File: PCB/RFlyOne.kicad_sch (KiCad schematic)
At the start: 21 parts, among them J1 UFL, Q1 AO3401A, U1 TQP3M9036, U2 TLV3201AIDBVR, U3 TA0970A, U4 TQP3M9036, U5 TA0970A

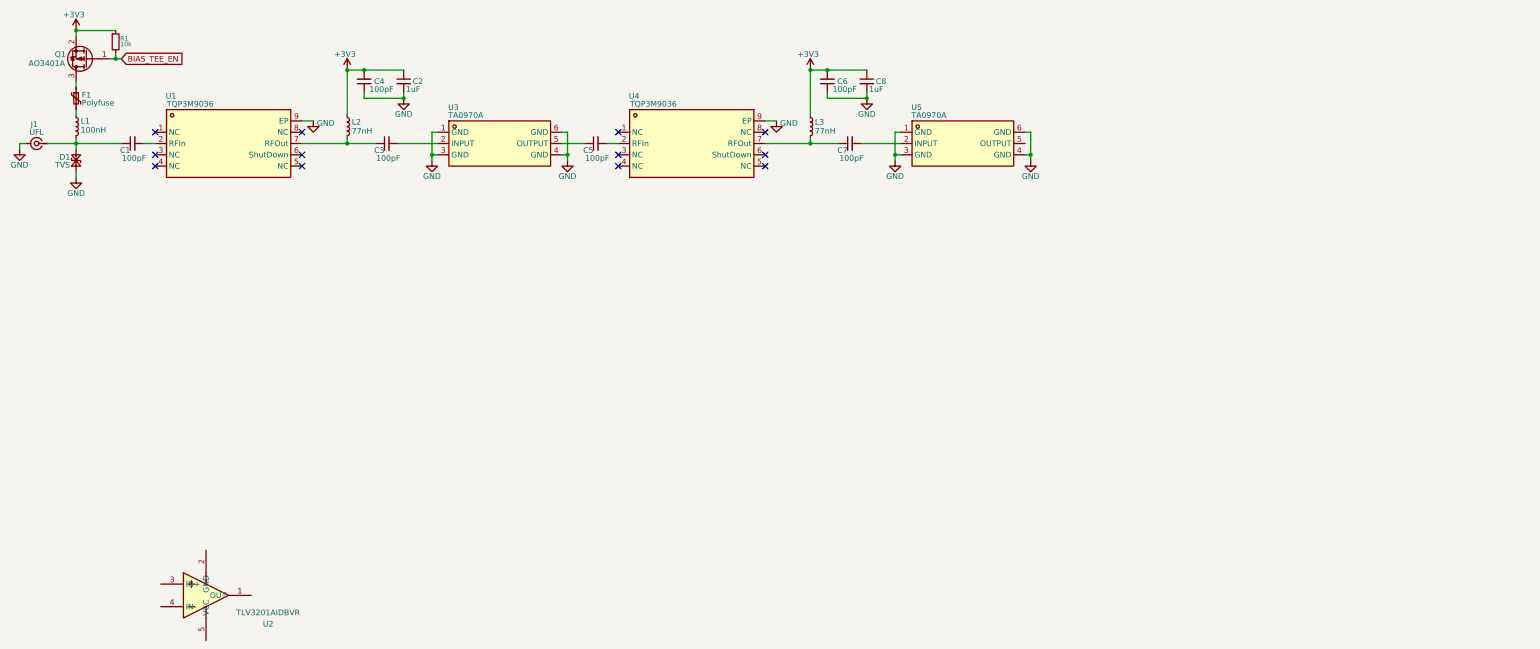
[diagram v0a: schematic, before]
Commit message: checkpoint
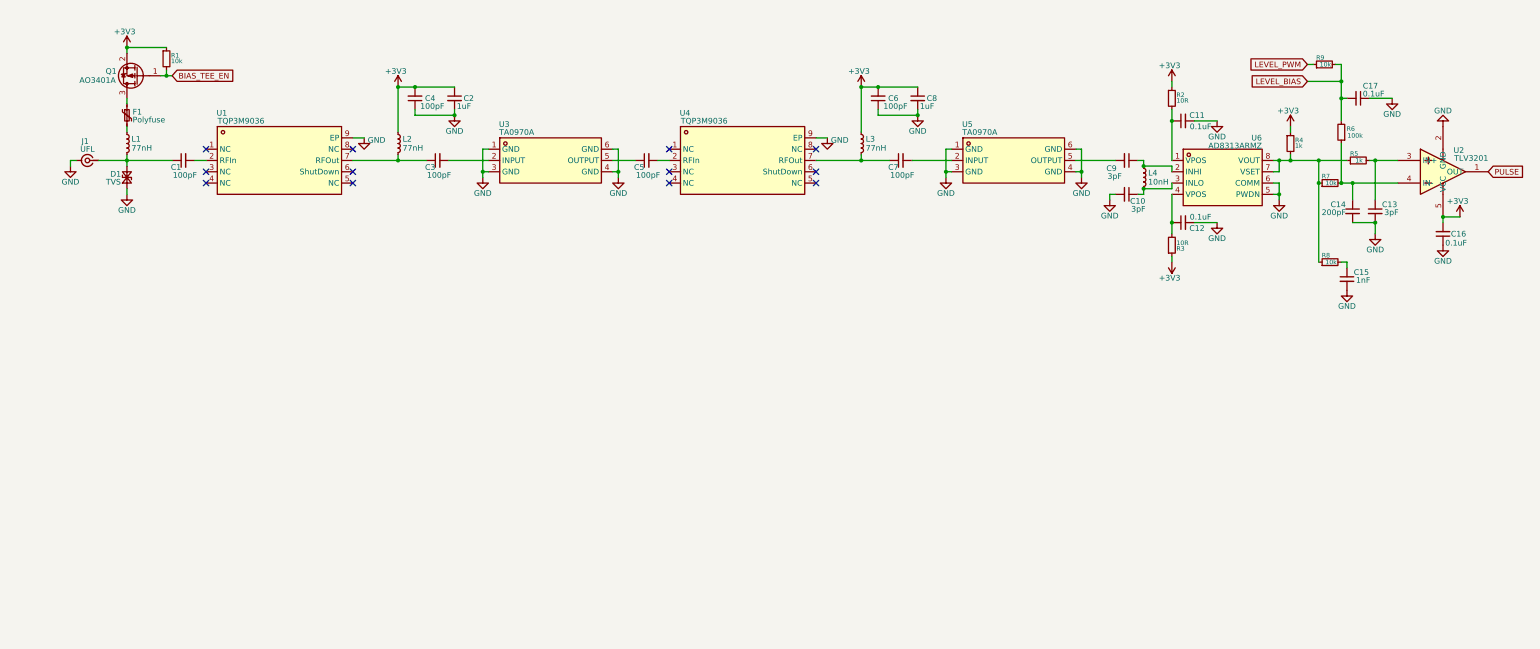
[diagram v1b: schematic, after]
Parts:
- added C10, C13, C9: 3pF, Capacitor_SMD:C_0402_1005Metric, symbol Device:C_Small
- added C11, C12, C16, C17: 0.1uF, Capacitor_SMD:C_0402_1005Metric, symbol Device:C_Small
- added C14: 200pF, Capacitor_SMD:C_0402_1005Metric, symbol Device:C_Small
- added C15: 1nF, Capacitor_SMD:C_0402_1005Metric, symbol Device:C_Small
- added L4: 10nH, Inductor_SMD:L_0402_1005Metric, symbol Device:L_Small
- added R2, R3: 10R, Resistor_SMD:R_0402_1005Metric, symbol Device:R_Small
- added R4, R5: 1k, Resistor_SMD:R_0402_1005Metric, symbol Device:R_Small
- added R6: 100k, Resistor_SMD:R_0402_1005Metric, symbol Device:R_Small
- added R7, R8, R9: 10k, Resistor_SMD:R_0402_1005Metric, symbol Device:R_Small
- added U6: AD8313ARMZ, easyeda2kicad:MSOP-8_L3.0-W3.0-P0.65-LS4.9-BL, symbol RFlyOne:AD8313ARMZ
- C1, C3, C4, C5, C6, C7: LCSC Part C1546 -> C77177
- L1: value 100nH -> 77nH; footprint easyeda2kicad:IND-SMD_L1.8-W1.2_LCF0603-150J-T -> Inductor_SMD:L_0402_1005Metric; LCSC Part C6808001 -> C668466
- Q1: LCSC Part (none) -> C15127; LCSC part C15127 -> (none)
- U2: value TLV3201AIDBVR -> TLV3201
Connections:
- net +3V3: now also U2.5 (VCC), C16.2, R2.1, R3.1, R4.1
- net GND: now also U2.2 (GND), C10.2, C11.2, C12.2, C13.2, C14.2, C15.2, C16.1, C17.1, U6.5 (PWDN), U6.6 (COMM)
- net at U5.5 (OUTPUT): now also C9.2
- net PULSE: now reaches U2.1 (OUT)
- net at U2.3 (IN+): now also C13.1, R5.2
- net at U2.4 (IN-): now also C14.1, R6.1, R7.2
- new net: R4.2, R5.1, R7.1, R8.1, U6.7 (VSET), U6.8 (VOUT)
- new net: C10.1, L4.2, U6.3 (INLO)
- new net: C9.1, L4.1, U6.2 (INHI)
- new net: C11.1, R2.2, U6.1 (VPOS)
- new net: C15.1, R8.2
- new net: C12.1, R3.2, U6.4 (VPOS)
- new net LEVEL_BIAS: C17.2, R6.2, R9.2
- new net LEVEL_PWM: R9.1
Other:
- moved on the sheet: C1, C2, C3, C4, C5, C6, C7, C8, D1, F1, J1, L2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
